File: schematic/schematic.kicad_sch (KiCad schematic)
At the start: 18 parts, among them J1 Conn_01x06, U1 ATmega328-PU

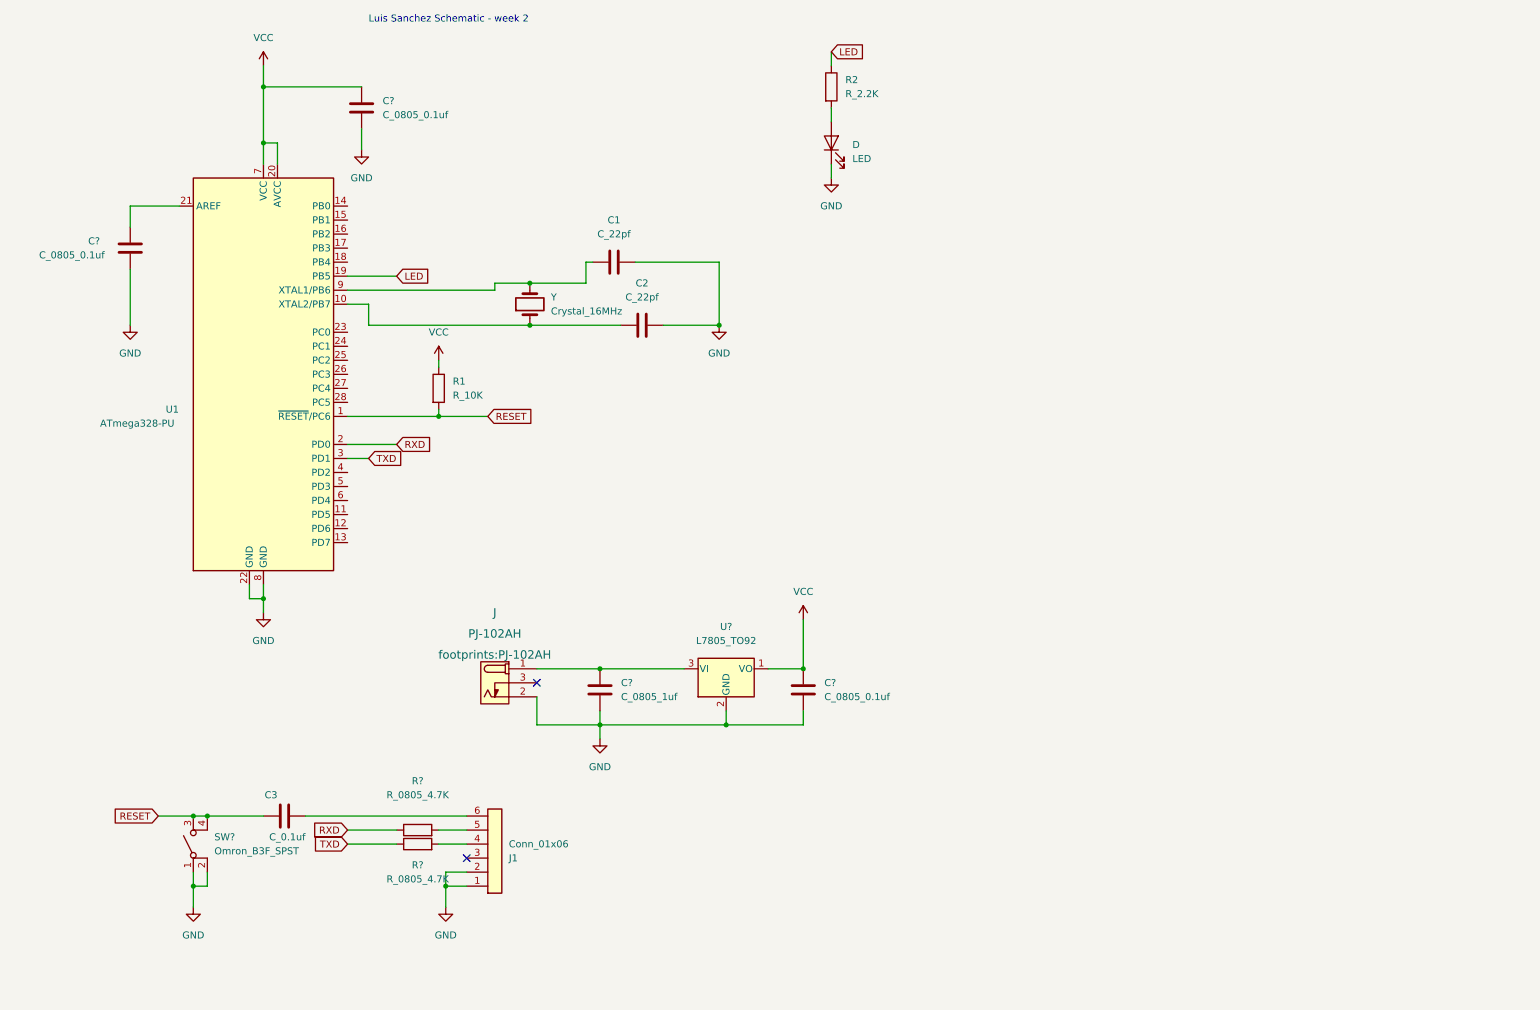
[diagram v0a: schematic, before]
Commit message: week 3 updates
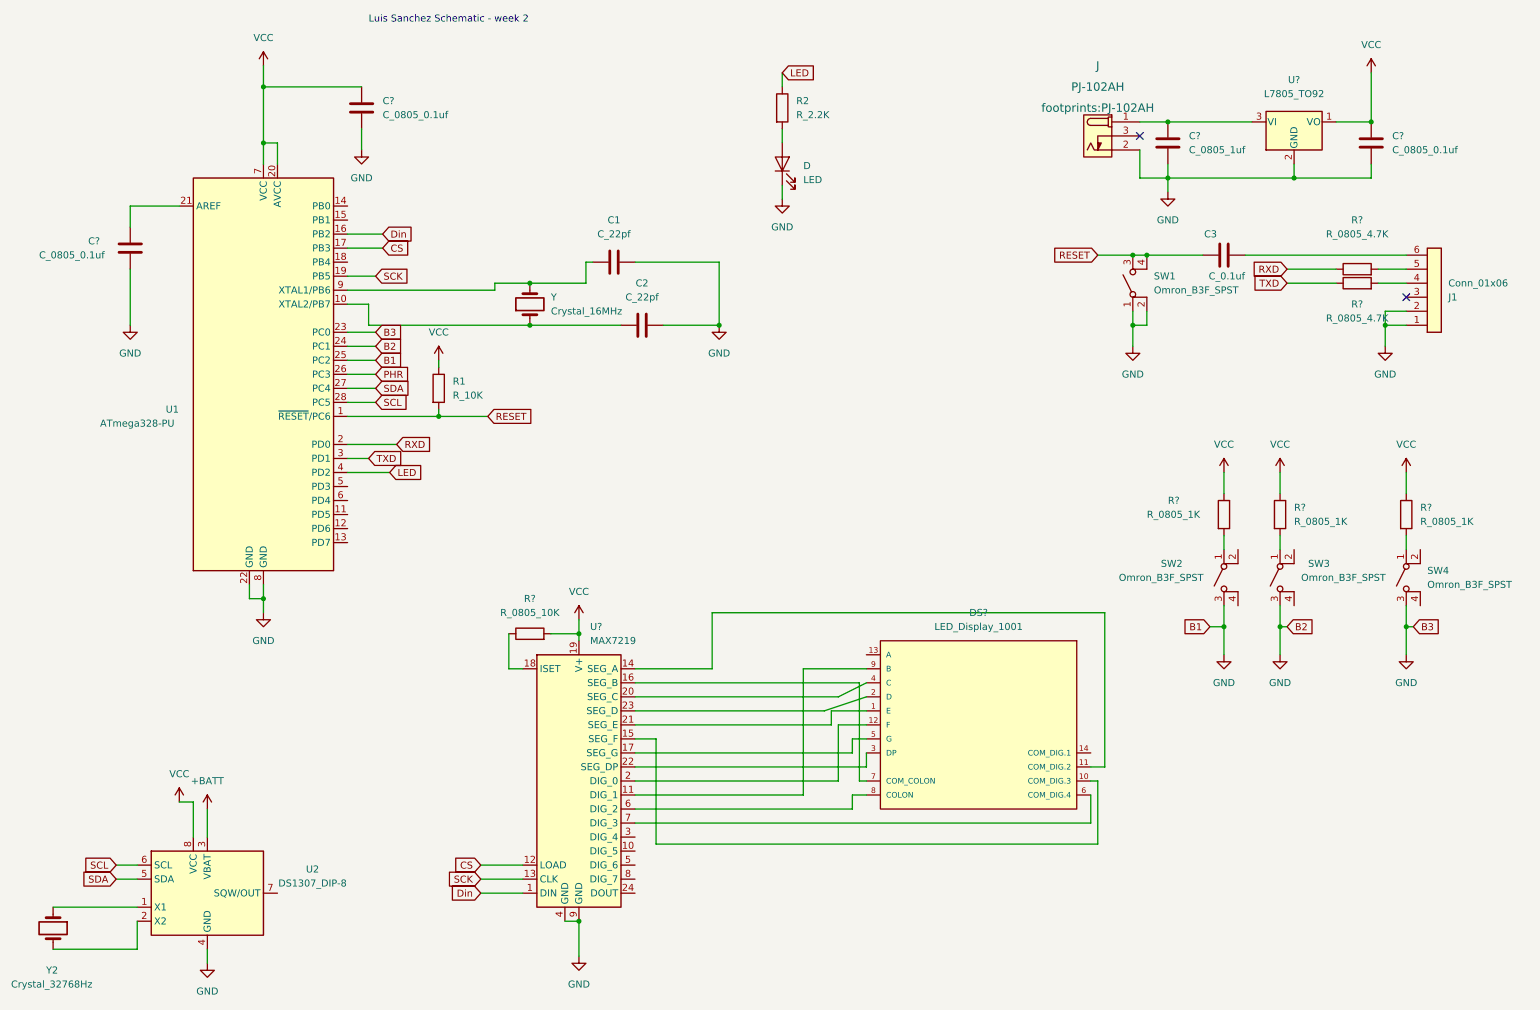
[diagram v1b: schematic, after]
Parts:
- added DS?: LED_Display_1001, footprints:Adafruit-1001-0-0-MFG, symbol HPS:LED_Display_1001
- added R?: R_0805_10K, footprints:R_0805_2012Metric, symbol HPS:R_0805_10K
- added R? (x3): R_0805_1K, footprints:R_0805_2012Metric, symbol HPS:R_0805_1K
- added SW2, SW3, SW4: Omron_B3F_SPST, footprints:SW_SPST_Omron_B3FS-100xP, symbol HPS:Omron_B3F_SPST
- added U2: DS1307_DIP-8, footprints:DIP-8_W7.62mm, symbol HPS:DS1307_DIP-8
- added U?: MAX7219, footprints:DIP-24_W7.62mm, symbol HPS:MAX7219
- added Y2: Crystal_32768Hz, footprints:Crystal_SMD_2Pin_3.2x1.5mm, symbol HPS:Crystal_32768Hz
- gave numbers to parts that had none: 1
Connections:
- net GND: now also U1.23 (PC0), U1.24 (PC1), U1.25 (PC2), SW2.3 (B), SW3.3 (B), SW4.3 (B), U2.4 (GND), U?.4 (GND), U?.9 (GND)
- net LED: now also U1.4 (PD2); no longer U1.19 (PB5)
- net VCC: now also R?.1, R?.1, R?.1, R?.2, U2.8 (VCC), U?.19 (V+)
- net Din: now reaches U1.16 (PB2)
- net Din: now also U?.1 (DIN)
- net CS: now reaches U1.17 (PB3)
- net CS: now also U?.12 (LOAD)
- net PHR: now reaches U1.26 (PC3)
- net SDA: now reaches U1.27 (PC4)
- net SDA: now also U2.5 (SDA)
- net SCL: now reaches U1.28 (PC5)
- net SCL: now also U2.6 (SCL)
- new net: R?.2, SW4.1 (A)
- new net: R?.2, SW2.1 (A)
- new net: R?.2, SW3.1 (A)
- new net: U2.1 (X1), Y2.1
- new net: U2.2 (X2), Y2.2
- new net: R?.1, U?.18 (ISET)
- new net: DS?.9 (B), U?.11 (DIG_1)
- new net: DS?.11 (COM_DIG.2), U?.14 (SEG_A)
- new net: DS?.10 (COM_DIG.3), U?.15 (SEG_F)
- new net: DS?.7 (COM_COLON), U?.16 (SEG_B)
- new net: DS?.5 (G), U?.17 (SEG_G)
- new net: DS?.12 (F), U?.2 (DIG_0)
- new net: DS?.4 (C), U?.20 (SEG_C)
- new net: DS?.1 (E), U?.21 (SEG_E)
- new net: DS?.3 (DP), U?.22 (SEG_DP)
- new net: DS?.2 (D), U?.23 (SEG_D)
- new net: DS?.8 (COLON), U?.6 (DIG_2)
- new net: DS?.6 (COM_DIG.4), U?.7 (DIG_3)
- new net +BATT: U2.3 (VBAT)
- new net SCK: U1.19 (PB5), U?.13 (CLK)
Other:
- moved on the sheet: C3, C?, D, J, J1, R2, R?, SW1, U?
